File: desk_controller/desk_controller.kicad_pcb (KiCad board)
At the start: 2 copper layers, 93.5 x 76.8 mm, 57 parts, among them J2 UART_passthrough, J3 SWD_header, J4 Barrel_Jack_MountingPin, J5 Barrel_Jack_MountingPin, SW2 STRIP_PWR_SW, SW3 PC_PWR_RST_SW, SW4 OS_SW, U1 BD95831MUV, U2 PC817, U3 AP2112K-3.3, U4 TRS3243ECRHBR, U5 ISO7341FC, U6 STM32F030K6T6, U7 PC817

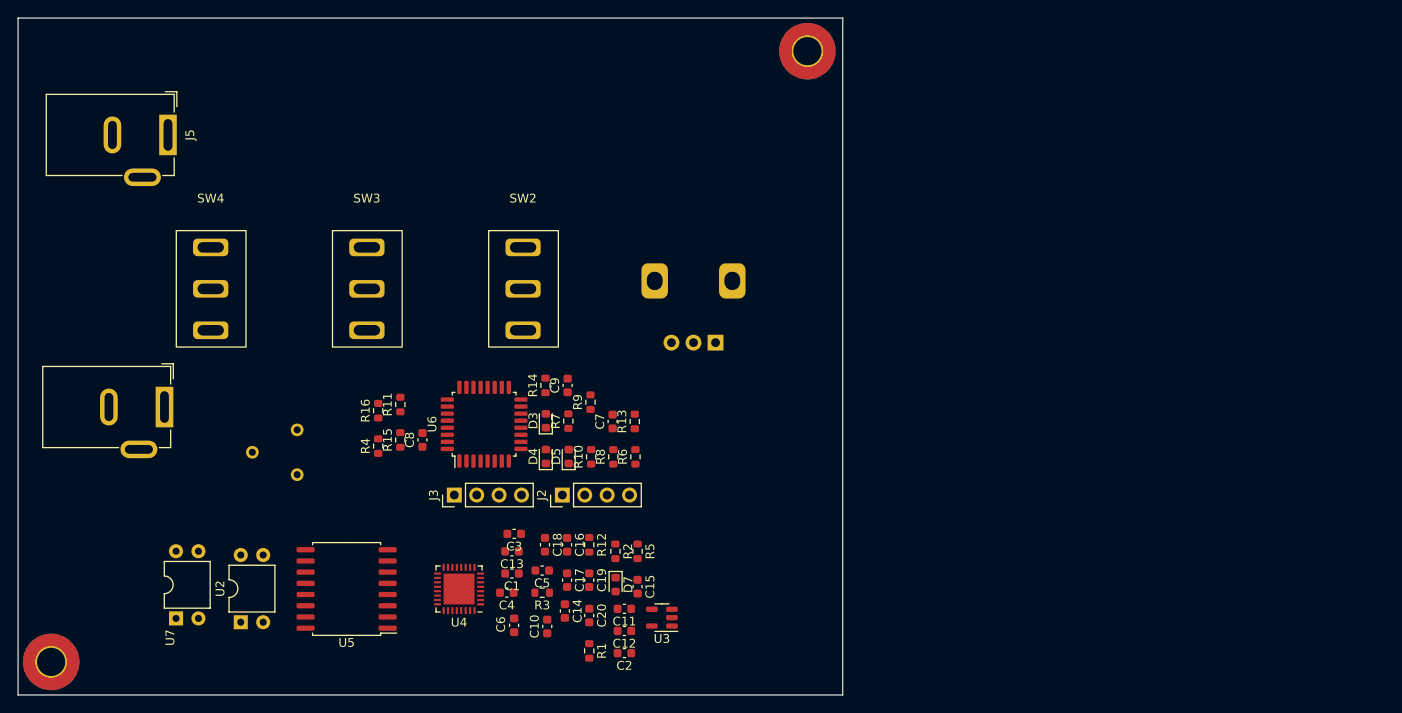
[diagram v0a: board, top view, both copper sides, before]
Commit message: Much progress in sch and brd
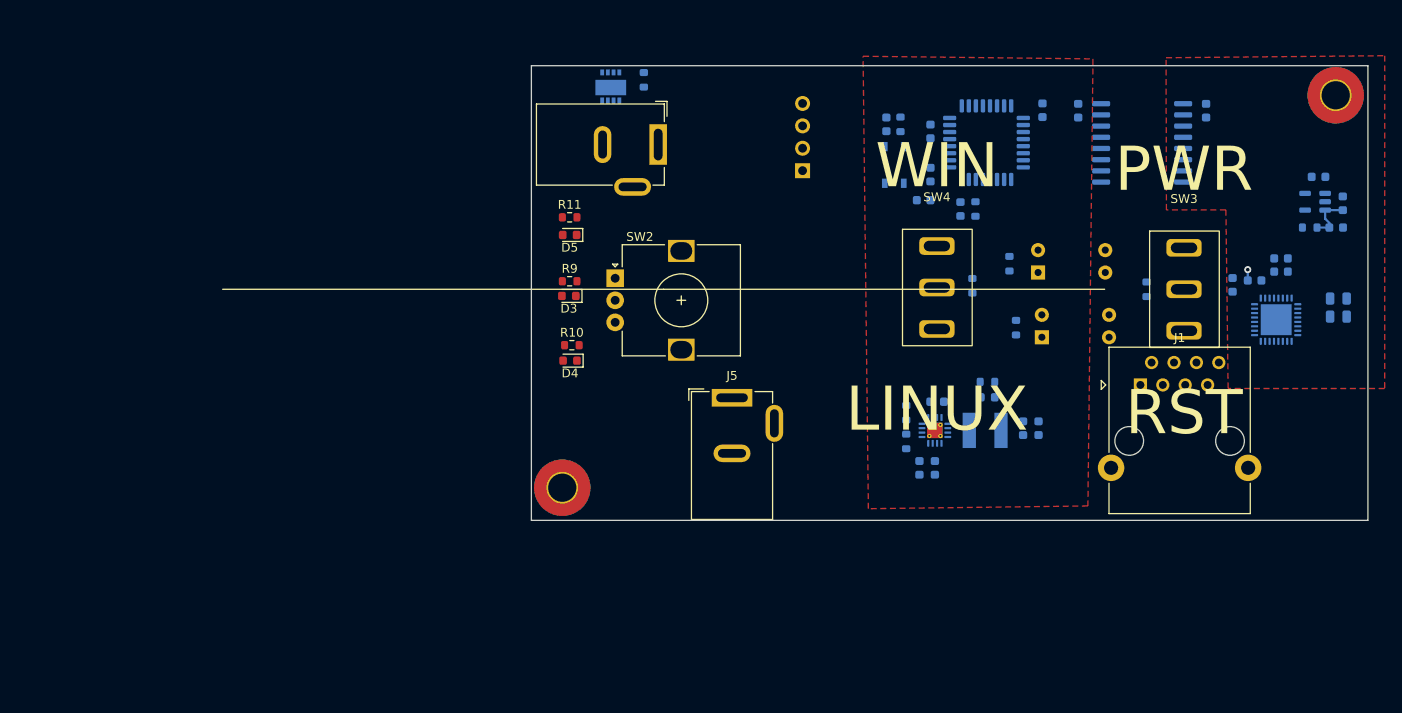
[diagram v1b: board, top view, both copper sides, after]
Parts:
- removed C20: 22u, Capacitor_SMD:C_0603_1608Metric
- removed J2: UART_passthrough, Connector_PinHeader_2.54mm:PinHeader_1x04_P2.54mm_Vertical
- removed R12: 3k3, Resistor_SMD:R_0603_1608Metric
- removed R16: 1k, Resistor_SMD:R_0603_1608Metric
- removed RV1: STRIP_BRIGTH, Potentiometer_THT:Potentiometer_Alps_RK09K_Single_Vertical
- added D1: D_Schottky, Diode_SMD:D_0805_2012Metric, B.Cu at (238.9, 75.5)
- added D2: D_Schottky, Diode_SMD:D_0805_2012Metric, B.Cu at (238.9, 77.6)
- added D6: RED, LED_SMD:LED_0603_1608Metric, B.Cu at (199.2, 86.8)
- added J1: RJ45, Connector_RJ:RJ45_Ninigi_GE, F.Cu at (216.5, 85.3)
- added L1: 4u7, BWVS005050404R7M00:BWVS005050404R7M00, B.Cu at (198.5, 90.5)
- added Q1: RQ3E110AJ, SOTFL65P330X80-8N:SOTFL65P330X80-8N, B.Cu at (156.4, 51.5)
- added SW1: SW_Push_Open_Dual, SKRPACE010:SW_SKRPACE010, B.Cu at (188.6, 60.4)
- C1, C10, C11, C12, C13, C14, C15, C19, C2, C3, C4, C5, C6, C7, C8, C9, D7, J3, R13, R14, R15, R3, R4, R6, R7, R8, U2, U3, U4, U5, U6, U7: moved to B.Cu
- C16: value 22n -> 100n; moved to B.Cu
- C17: value 10u -> 22n; moved to B.Cu
- C18: value 1n -> 22u; moved to B.Cu
- R1: value 4k7 -> 10k; moved to B.Cu
- R2: value 1k5 -> 3k7; moved to B.Cu
- R5: value 13k -> 1k; moved to B.Cu
- SW2: value STRIP_PWR_SW -> RotaryEncoder; footprint MTS-102-103:MTS-102-103 -> Rotary_Encoder:RotaryEncoder_Alps_EC12E_Vertical_H20mm
- U1: value BD95831MUV -> TS30042-M000QFNR; footprint Potentiometer_THT:Potentiometer_Bourns_3386F_Vertical -> Package_DFN_QFN:QFN-16-1EP_3x3mm_P0.5mm_EP1.75x1.75mm_ThermalVias
- moved U5 103.4 mm to (216.7, 57.9)
- moved U7 103.2 mm to (205.3, 79.9), turned to 0 degrees
- moved C1 101.4 mm to (238.7, 67.5), turned to 0 degrees
- moved C3 99.8 mm to (236.7, 61.8), turned to 0 degrees
- moved U2 98.7 mm to (204.9, 72.6), turned to 0 degrees
- moved U4 97.6 mm to (231.9, 78.0)
- moved R3 96.4 mm to (235.7, 67.5)
- moved C4 96.3 mm to (223.9, 54.2), turned to -90 degrees
- moved C2 96.1 mm to (239.4, 64.8), turned to 90 degrees
- moved SW3 92.7 mm to (221.4, 74.5)
- moved C14 89.9 mm to (232.4, 72.5), turned to 0 degrees
- moved U3 87.8 mm to (236.3, 64.6)
- moved C13 87.1 mm to (226.9, 74.0), turned to -90 degrees
- moved C12 85.6 mm to (232.4, 71.0), turned to 0 degrees
- moved SW4 82.3 mm to (193.4, 74.3)
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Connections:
- net GND2 renamed PC_GND
- C15 pad 1: +12V -> GND
- C15 pad 2: GND -> +12V
- C16 pad 2: Net-(C16-Pad2) -> +12V
- C17 pad 1: GND -> Net-(C17-Pad1)
- C17 pad 2: +12V -> Net-(C17-Pad2)
- C18 pad 1: Net-(C18-Pad1) -> GND
- C18 pad 2: Net-(C18-Pad2) -> +3V3
- C19 pad 2: +3.3V -> +3V3
- C5 pad 1: Net-(C5-Pad1) -> GND
- R1 pad 1: Net-(R1-Pad1) -> +3V3
- R1 pad 2: GND -> Net-(R1-Pad2)
- R2 pad 1: Net-(R1-Pad1) -> Net-(R1-Pad2)
- R2 pad 2: Net-(R2-Pad2) -> GND
- R5 pad 1: Net-(R2-Pad2) -> Net-(D6-Pad2)
- R5 pad 2: +3.3V -> +3V3
- U1 pad 1: +12V -> Net-(C17-Pad2)
- U1 pad 3: GND -> +12V
- U2 pad 4: /mcu/POWER+ -> POWER
- U4 pad 12: TTL_RX -> /rs232/TTL_RX
- U4 pad 15: TTL_RTS -> /rs232/TTL_RTS
- U4 pad 17: TTL_DTR -> /rs232/TTL_DTR
- U4 pad 18: TTL_TX -> /rs232/TTL_TX
- U5 pad 11: TTL_RX -> TTL_RX_ISO
- U5 pad 12: TTL_RTS -> TTL_RTS_ISO
- U5 pad 13: TTL_DTR -> TTL_DTR_ISO
- U5 pad 14: TTL_TX -> TTL_TX_ISO
- U5 pad 15: Net-(C5-Pad1) -> GND
- U5 pad 3: /rs232/232_TX -> /rs232/TTL_TX
- U5 pad 4: /rs232/232_DTR -> /rs232/TTL_DTR
- U5 pad 5: /rs232/232_RTS -> /rs232/TTL_RTS
- U5 pad 6: /rs232/232_RX -> /rs232/TTL_RX
- U5 pad 9: Net-(C5-Pad1) -> GND
- U6 pad 10: unconnected-(U6-Pad10) -> TTL_TX_ISO
- U6 pad 11: unconnected-(U6-Pad11) -> TTL_DTR_ISO
- U6 pad 12: unconnected-(U6-Pad12) -> TTL_RTS_ISO
- U6 pad 13: unconnected-(U6-Pad13) -> TTL_RX_ISO
- U7 pad 4: /mcu/RESET+ -> RESET
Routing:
- net /rs232/232_VUR: track 0.00 -> 5.57 mm
- net GND1: track 0.00 -> 1.22 mm, vias 0 -> 1
- added copper zone on F.Cu, net GND
- added copper zone on F.Cu, net GND1
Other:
- board size 93.5 x 76.8 mm -> 94.9 x 51.6 mm
- board text added: "LINUX"
- board text added: "PWR"
- board text added: "RST"
- board text added: "WIN"
